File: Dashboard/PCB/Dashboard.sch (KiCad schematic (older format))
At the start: 97 parts, among them J3 LED, J4 MAIN_CONNECTOR, J5 BAOFENG_OUT, J6 Display, J7 PROGRAMMER, J8 MEM2051-00-195-00-A_REVC, SW1 SW_SPST, U1 STM32F767ZIT6, U2 MP2359DJ-LF-Z, U3 MP2359DJ-LF-Z, U4 AS4C1M16S-6TCN, U5 AT25SF128A-SHB-T, U6 MP2332H, U7 MCP2561-E-SN, U8 MCP2561-E-SN, Y1 Crystal_GND24

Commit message: Remove unnecessary files
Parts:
- removed J8: MEM2051-00-195-00-A_REVC, SDCARD:GCT_MEM2051-00-195-00-A_REVC, symbol MEM2051-00-195-00-A_REVC:MEM2051-00-195-00-A_REVC
- removed R19, R20, R21, R22: 47K, Resistor_SMD:R_0805_2012Metric, symbol Device:R
- added U?: ESP-12S, ESP-12S, symbol ESP-12S:ESP-12S
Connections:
- wire segments 405 -> 388
- no-connect marks 62 -> 70
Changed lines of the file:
@@
 	10950 13500 11050 13600
 Entry Wire Line
-	20500 5400 20600 5500
-Entry Wire Line
 	14550 12400 14650 12500
 $Comp
@@
 	12750 12300 12750 11700
 Connection ~ 12750 11700
-$Comp
-L power:+3.3V #PWR061
-U 1 1 61E60003
-P 13350 9250
-F 0 "#PWR061" H 13350 9100 50  0001 C CNN
-F 1 "+3.3V" H 13365 9423 50  0000 C CNN
-F 2 "" H 13350 9250 50  0001 C CNN
-F 3 "" H 13350 9250 50  0001 C CNN
-	1    13350 9250
-	-1   0    0    -1
-$EndComp
-$Comp
-L power:GND #PWR062
-U 1 1 61E60BC0
-P 13350 9950
-F 0 "#PWR062" H 13350 9700 50  0001 C CNN
-F 1 "GND" H 13355 9777 50  0000 C CNN
-F 2 "" H 13350 9950 50  0001 C CNN
-F 3 "" H 13350 9950 50  0001 C CNN
-	1    13350 9950
-	-1   0    0    -1
-$EndComp
-Wire Wire Line
-	13050 9950 13350 9950
-Wire Wire Line
-	13350 9250 13050 9250
-Entry Wire Line
-	13900 9650 14000 9750
-Entry Wire Line
-	13900 9750 14000 9850
-Entry Wire Line
-	13900 9350 14000 9450
-NoConn ~ 13050 9450
-NoConn ~ 13050 9550
-Entry Wire Line
-	13900 9850 14000 9950
-Text Label 13100 9350 0    50   ~ 0
-SD_MISO
-Text Label 13100 9850 0    50   ~ 0
-SD_SCLK
-Text Label 13100 9750 0    50   ~ 0
-SD_MOSI
-Text Label 13150 9650 0    50   ~ 0
-SD_CS
-$Comp
-L power:GND #PWR060
-U 1 1 61F62558
-P 13050 10250
-F 0 "#PWR060" H 13050 10000 50  0001 C CNN
-F 1 "GND" H 13055 10077 50  0000 C CNN
-F 2 "" H 13050 10250 50  0001 C CNN
-F 3 "" H 13050 10250 50  0001 C CNN
-	1    13050 10250
-	1    0    0    -1
-$EndComp
 Wire Wire Line
 	15200 12500 14650 12500
@@
 Entry Wire Line
 	13150 1850 13050 1950
-$Comp
-L Device:R R22
-U 1 1 6240A074
-P 13900 9050
-F 0 "R22" H 13970 9096 50  0000 L CNN
-F 1 "47K" H 13970 9005 50  0000 L CNN
-F 2 "Resistor_SMD:R_0805_2012Metric" V 13830 9050 50  0001 C CNN
-F 3 "~" H 13900 9050 50  0001 C CNN
-	1    13900 9050
-	1    0    0    -1
-$EndComp
-$Comp
-L Device:R R21
-U 1 1 6249BF7E
-P 13800 9050
-F 0 "R21" H 13870 9096 50  0000 L CNN
-F 1 "47K" H 13870 9005 50  0000 L CNN
-F 2 "Resistor_SMD:R_0805_2012Metric" V 13730 9050 50  0001 C CNN
-F 3 "~" H 13800 9050 50  0001 C CNN
-	1    13800 9050
-	1    0    0    -1
-$EndComp
-$Comp
-L Device:R R20
-U 1 1 624ABC5A
-P 13700 9050
-F 0 "R20" H 13770 9096 50  0000 L CNN
-F 1 "47K" H 13770 9005 50  0000 L CNN
-F 2 "Resistor_SMD:R_0805_2012Metric" V 13630 9050 50  0001 C CNN
-F 3 "~" H 13700 9050 50  0001 C CNN
-	1    13700 9050
-	1    0    0    -1
-$EndComp
-$Comp
-L Device:R R19
-U 1 1 624ABC60
-P 13600 9050
-F 0 "R19" H 13670 9096 50  0000 L CNN
-F 1 "47K" H 13670 9005 50  0000 L CNN
-F 2 "Resistor_SMD:R_0805_2012Metric" V 13530 9050 50  0001 C CNN
-F 3 "~" H 13600 9050 50  0001 C CNN
-	1    13600 9050
-	1    0    0    -1
-$EndComp
-Wire Wire Line
-	13900 9200 13900 9350
-Wire Wire Line
-	13900 8900 13800 8900
-Connection ~ 13700 8900
-Wire Wire Line
-	13700 8900 13600 8900
-Connection ~ 13800 8900
-Wire Wire Line
-	13800 8900 13700 8900
-$Comp
-L power:+3.3V #PWR063
-U 1 1 62568F6D
-P 13600 8900
-F 0 "#PWR063" H 13600 8750 50  0001 C CNN
-F 1 "+3.3V" H 13615 9073 50  0000 C CNN
-F 2 "" H 13600 8900 50  0001 C CNN
-F 3 "" H 13600 8900 50  0001 C CNN
-	1    13600 8900
-	1    0    0    -1
-$EndComp
-Connection ~ 13600 8900
-Wire Bus Line
-	14000 9950 14550 9950
-Connection ~ 14550 9950
 NoConn ~ 12350 1850
 NoConn ~ 12350 2050
 NoConn ~ 12350 2150
 NoConn ~ 13200 7850
-$Comp
-L MEM2051-00-195-00-A_REVC:MEM2051-00-195-00-A_REVC J8
-U 1 1 617876F8
-P 12850 9750
-F 0 "J8" H 13480 9796 50  0000 L CNN
-F 1 "MEM2051-00-195-00-A_REVC" H 13480 9705 50  0000 L CNN
-F 2 "SDCARD:GCT_MEM2051-00-195-00-A_REVC" H 12850 9750 50  0001 L BNN
-F 3 "" H 12850 9750 50  0001 L BNN
-F 4 "GCT" H 12850 9750 50  0001 L BNN "MANUFACTURER"
-	1    12850 9750
-	-1   0    0    -1
-$EndComp
-Wire Wire Line
-	13050 9650 13800 9650
-Wire Wire Line
-	13050 9350 13900 9350
-Wire Wire Line
-	13050 9750 13700 9750
-Wire Wire Line
-	13050 9850 13600 9850
-Wire Wire Line
-	13800 9200 13800 9650
-Connection ~ 13800 9650
-Wire Wire Line
-	13800 9650 13900 9650
-Wire Wire Line
-	13700 9200 13700 9750
-Connection ~ 13700 9750
-Wire Wire Line
-	13700 9750 13900 9750
-Wire Wire Line
-	13600 9200 13600 9850
-Connection ~ 13600 9850
-Wire Wire Line
-	13600 9850 13900 9850
-Wire Wire Line
-	13050 10150 13900 10150
-Wire Bus Line
-	14000 9950 14000 10250
-Connection ~ 14000 9950
-Entry Wire Line
-	13900 10150 14000 10250
-Text Label 13100 10150 0    50   ~ 0
-SD_CARD_DETECT
 Entry Wire Line
 	14550 1300 14650 1400
@@
 	4550 14850 4550 14750
 Connection ~ 4550 14850
-Wire Notes Line
-	900  800  3800 800
-Text Notes 1150 750  2    50   ~ 0
+Text Notes 1050 700  2    50   ~ 0
 Power\n
 Wire Notes Line
-	3800 4200 900  4200
-Wire Notes Line
-	900  800  900  4200
-Wire Notes Line
-	3800 800  3800 4200
-Wire Notes Line
 	4300 5300 9050 5300
 Wire Notes Line
@@
 Wire Wire Line
 	4550 6750 4550 6900
+$Comp
+L ESP-12S:ESP-12S U?
+U 1 1 61B531D3
+P 10550 7550
+F 0 "U?" H 10550 8417 50  0000 C CNN
+F 1 "ESP-12S" H 10550 8326 50  0000 C CNN
+F 2 "ESP-12S" H 10550 7550 50  0001 L BNN
+F 3 "" H 10550 7550 50  0001 L BNN
+F 4 "IC-14115" H 10550 7550 50  0001 L BNN "PROD_ID"
+	1    10550 7550
+	1    0    0    -1
+$EndComp
+NoConn ~ 10950 7150
+NoConn ~ 10950 7250
+NoConn ~ 10950 7350
+NoConn ~ 10950 7450
+NoConn ~ 10950 7550
+NoConn ~ 10950 7650
+NoConn ~ 10950 7750
+NoConn ~ 10950 7850
+NoConn ~ 10950 7950
+NoConn ~ 10950 8050
 Wire Bus Line
 	13150 1350 13150 1550
 Wire Bus Line
-	14000 9450 14000 9950
-Wire Bus Line
 	14200 7350 14200 7950
 Wire Bus Line
@@
 	13150 1550 13150 2250
 Wire Bus Line
-	14550 7950 14550 9950
-Wire Bus Line
 	14550 1550 14550 7950
 Wire Bus Line
 	10950 11400 10950 14000
 Wire Bus Line
-	14550 9950 14550 14000
-Wire Bus Line
 	13350 11600 13350 14000
+Wire Bus Line
+	14550 7950 14550 14000
+$Comp
+L power:+3.3V #PWR?
+U 1 1 61E1DAA6
+P 10050 6950
+F 0 "#PWR?" H 10050 6800 50  0001 C CNN
+F 1 "+3.3V" H 10065 7123 50  0000 C CNN
+F 2 "" H 10050 6950 50  0001 C CNN
+F 3 "" H 10050 6950 50  0001 C CNN
+	1    10050 6950
+	1    0    0    -1
+$EndComp
 $EndSCHEMATC

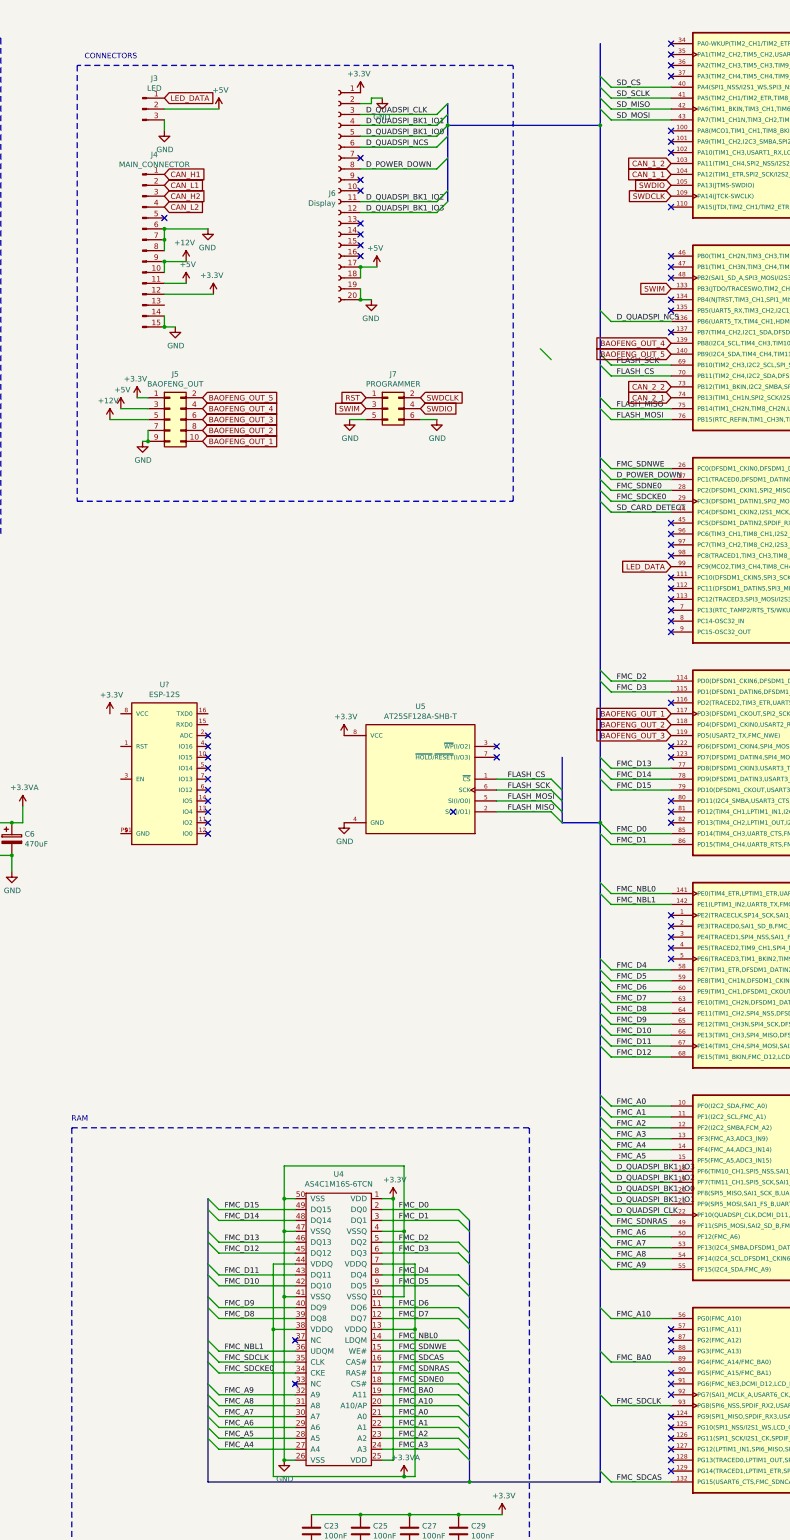
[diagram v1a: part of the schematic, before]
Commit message: ADD new pcb files
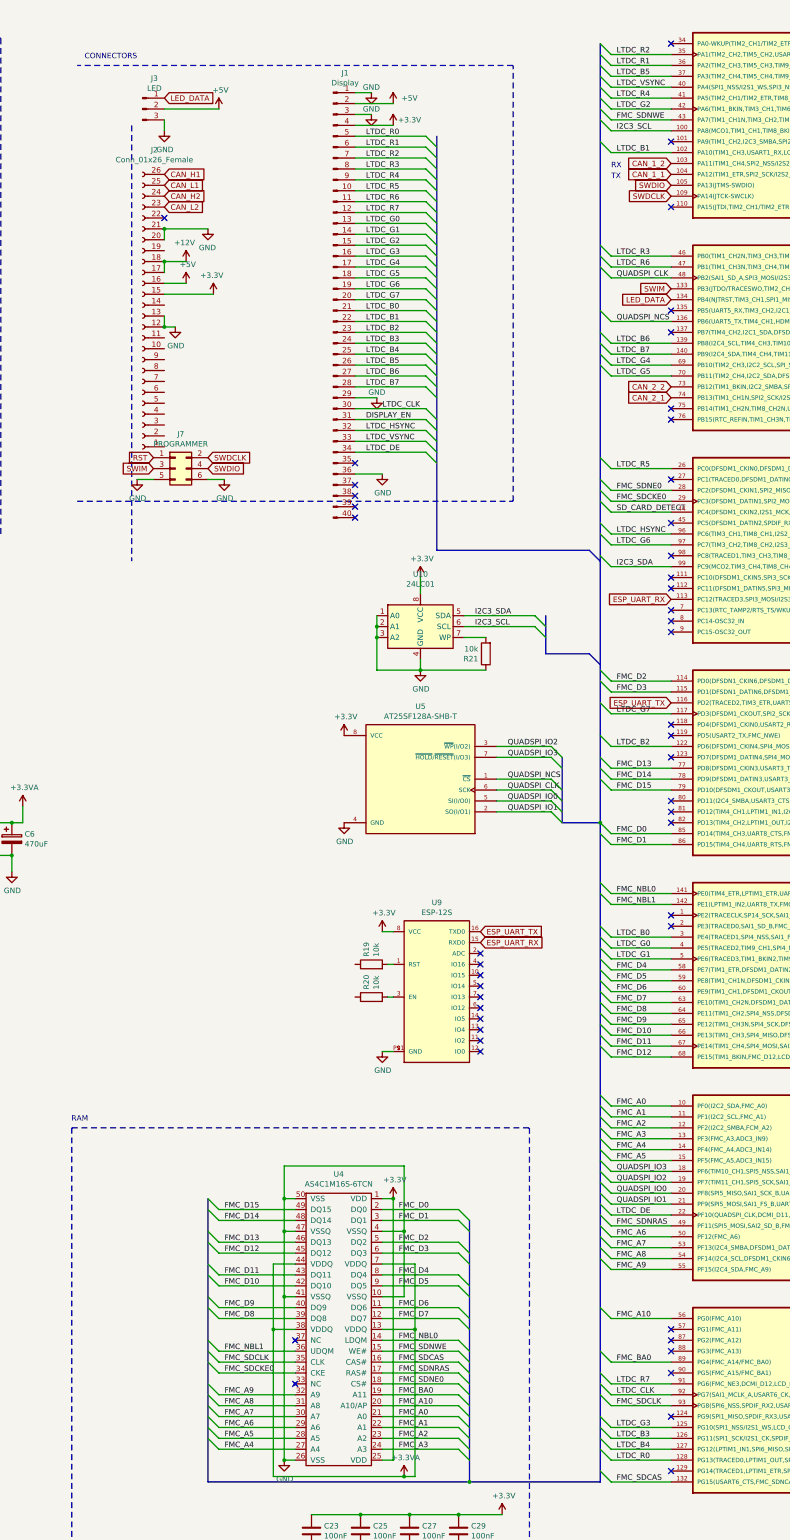
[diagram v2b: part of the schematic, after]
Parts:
- removed J4: MAIN_CONNECTOR, Connector:DT13, symbol Connector:Conn_01x15_Male
- removed J5: BAOFENG_OUT, Connector_PinSocket_2.54mm:PinSocket_2x05_P2.54mm_Vertical, symbol Connector_Generic:Conn_02x05_Odd_Even
- removed J6: Display, Connector_FFC-FPC:Hirose_FH12-20S-0.5SH_1x20-1MP_P0.50mm_Horizontal, symbol Connector:Conn_01x20_Female
- added J1: Display, Connector_FFC-FPC:Hirose_FH12-40S-0.5SH_1x40-1MP_P0.50mm_Horizontal, symbol Connector:Conn_01x40_Male
- added J2: Conn_01x26_Female, Konektor:64734231, symbol Connector:Conn_01x26_Female
- added R19, R20, R21: 10k, Resistor_SMD:R_0805_2012Metric, symbol Device:R
- added U10: 24LC01, Package_DIP:DIP-8_W7.62mm_Socket_LongPads, symbol Memory_EEPROM:24LC01
- U9: renamed from U?; footprint ESP-12S -> ESP-12S:ESP-12S
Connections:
- net D_QUADSPI_BK1_IO2 is gone; now on net QUADSPI_IO2: U1.19 (PF7(TIM11_CH1,SPI5_SCK,SAI1_MCK_B,UART7_TX,QUADSPI_BK1_IO2,ADC3_IN5))
- net D_QUADSPI_BK1_IO3 is gone; now on net QUADSPI_IO3: U1.18 (PF6(TIM10_CH1,SPI5_NSS,SAI1_SD_B,UART7_RX,QUADSPI_BK1_IO3,ADC3_IN4))
- net SD_MOSI is gone; now on net FMC_SDNWE: U1.43 (PA7(TIM1_CH1N,TIM3_CH2,TIM8_CH1N,SPI1_MOSI/I2S1_SD,SPI6_MOSI,TIM14_CH1,ETH_MII_RX_DV/ETH_RMII_CRS_DV,FMC_SDNWE))
- net +12V: now also J2.17 (Pin_17), J2.18 (Pin_18)
- net +3V3: now also U9.8 (VCC), J1.4 (Pin_4), J2.15 (Pin_15), U10.8 (VCC)
- net +5V: now also J1.2 (Pin_2), J2.16 (Pin_16)
- net CAN_H1: now also J2.26 (Pin_26)
- net CAN_H2: now also J2.24 (Pin_24)
- net CAN_L1: now also J2.25 (Pin_25)
- net CAN_L2: now also J2.23 (Pin_23)
- net FMC_SDNWE: no longer U1.26 (PC0(DFSDM1_CKIN0,DFSDM1_DATIN4,SAI2_FS_B,OTG_HS_ULPI_STP,FMC_SDNWE,LCD_R5,ADC1_IN10,ADC2_IN10,ADC3_IN10))
- net GND: now also U9.9 (GND), U9.P$1 (GND), J1.1 (Pin_1), J1.29 (Pin_29), J1.3 (Pin_3), J1.36 (Pin_36), J2.12 (Pin_12), J2.13 (Pin_13), J2.20 (Pin_20), J2.21 (Pin_21), R21.1, U10.1 (A0), U10.2 (A1), U10.3 (A2), U10.4 (GND)
- net LED_DATA: now also U1.134 (PB4(NJTRST,TIM3_CH1,SPI1_MISO,SPI3_MISO,SPI2_NSS/I2S2_WS,SPI6_MISO,SDMMC2_D3,CAN3_TX,UART7_TX)); no longer U1.99 (PC9(MCO2,TIM3_CH4,TIM8_CH4,I2S3_SDA,I2S_CKIN,UART5_CTS,QUADSPI_BK1_IO0,LCD_G3,SDMMC12_D1,DCMI_D3,LCD_B2))
- net I2C3_SCL: now reaches U1.100 (PA8(MCO1,TIM1_CH1,TIM8_BKIN2,I2C3_SCL,USART1_CK,OTG_FS_SOF,CAN3_RX,UART7_RX,LCD_B3,LCD_R6))
- net I2C3_SCL: now also U10.6 (SCL)
- net LTDC_B1: now reaches U1.102 (PA10(TIM1_CH3,USART1_RX,LCD_B4,OTG_FS_ID,MDIOS_MDIO,DCMI_D1,LCD_B1))
- net LTDC_B1: now also J1.22 (Pin_22)
- net LTDC_R2: now reaches U1.35 (PA1(TIM2_CH2,TIM5_CH2,USART2_RTS,UART4_RX,QUADSPI_BK1_IO3,SAI2_MCLK_B,ETH_MII_RX_CLK/ETH_RMII_REF_CLK,LCD_R2))
- net LTDC_R2: now also J1.7 (Pin_7)
- net LTDC_R1: now reaches U1.36 (PA2(TIM2_CH3,TIM5_CH3,TIM9_CH1,USART2_TX,SAI2_SCK_B,ETH_MDIO,MDIOS_MDIO,LCD_R1,ADC1_IN2,ADC2_IN2,ADC3_IN2,WKUP2))
- net LTDC_R1: now also J1.6 (Pin_6)
- net LTDC_B5: now reaches U1.37 (PA3(TIM2_CH4,TIM5_CH4,TIM9_CH2,USART2_RX,LCD_B2,OTG_HS_ULPI_D0,ETH_MII_COL,LCD_B5,ADC1_IN3,ADC2_IN3,ADC3_IN3))
- net LTDC_B5: now also J1.26 (Pin_26)
- net LTDC_R3: now reaches U1.46 (PB0(TIM1_CH2N,TIM3_CH3,TIM8_CH2N,DFSDM1_CKOUT,UART4_CTS,LCD_R3,OTG_HS_ULPI_D1,ETH_MII_RXD2,LCD_G1,ADC1_IN8,ADC2_IN8))
- net LTDC_R3: now also J1.8 (Pin_8)
- net LTDC_R6: now reaches U1.47 (PB1(TIM1_CH3N,TIM3_CH4,TIM8_CH3N,DFSDM1_DATIN1,LCD_R6,OTG_HS_ULPI_D2,ETH_MII_RXD3,LCD_G0,ADC1_IN9,ADC2_IN9))
- net LTDC_R6: now also J1.11 (Pin_11)
- net QUADSPI_CLK: now reaches U1.48 (PB2(SAI1_SD_A,SPI3_MOSI/I2S3_SD,QUADSPI_CLK,DFSDM1_CKIN1))
- net QUADSPI_CLK: now also U5.6 (SCK)
- net ESP_UART_RX: now reaches U1.113 (PC12(TRACED3,SPI3_MOSI/I2S3_SD,USART3_CK,UART5_TX,SDMMC1_CK,DCMI_D9))
- net ESP_UART_RX: now also U9.15 (RXD0)
- net LTDC_HSYNC: now reaches U1.96 (PC6(TIM3_CH1,TIM8_CH1,I2S2_MCK,DFSDM1_CKIN3,USART6_TX,TMC_NWAIT,SDMMC2_D6,SDMMC1_D6,DCMI_D0,LCD_HSYNC))
- net LTDC_HSYNC: now also J1.32 (Pin_32)
- net LTDC_G6: now reaches U1.97 (PC7(TIM3_CH2,TIM8_CH2,I2S3_MCK,DFSDM1_DATIN3,USART6_RX,FMC_NE1,SDMMC2_D7,SDMMC1_D7,DCMI_D1,LCD_G6))
- net LTDC_G6: now also J1.19 (Pin_19)
- net ESP_UART_TX: now reaches U1.116 (PD2(TRACED2,TIM3_ETR,UART5_RX,SDMMC1_CMD,DCMI_D11))
- net ESP_UART_TX: now also U9.16 (TXD0)
- net LTDC_B2: now reaches U1.122 (PD6(DFSDM1_CKIN4,SPI4_MOSI/I2S3_SD,SAI1_SD_A,USART2_RX,DFSDM1_DATIN1,SDMMC2_CK,FMC_NWAIT,DCMI_D10,LCD_B2))
- net LTDC_B2: now also J1.23 (Pin_23)
- net LTDC_B0: now reaches U1.3 (PE4(TRACED1,SPI4_NSS,SAI1_FS_A,DFSDM1_DATIN3,FMC_A20,DCMI_D4,LCD_B0))
- net LTDC_B0: now also J1.21 (Pin_21)
- net LTDC_G0: now reaches U1.4 (PE5(TRACED2,TIM9_CH1,SPI4_MISO,SAI1_SCK_A,DFSDM1_CKIN3,FMC_A21,DCMI_D6,LCD_G0))
- net LTDC_G0: now also J1.13 (Pin_13)
- net LTDC_G1: now reaches U1.5 (PE6(TRACED3,TIM1_BKIN2,TIM9_CH2,SPI4_MOSI,SAI1_SD_A,SAI2_MCLK_B,FMC_A22,DCMI_D7,LCD_G1))
- net LTDC_G1: now also J1.14 (Pin_14)
- net LTDC_G3: now reaches U1.125 (PG10(SPI1_NSS/I2S1_WS,LCD_G3,SAI2_SD_B,SDMMC2_D1,FMC_NE3,DCMI_D2,LCD_B2))
- net LTDC_G3: now also J1.16 (Pin_16)
- net LTDC_B3: now reaches U1.126 (PG11(SPI1_SCK/I2S1_CK,SPDIF_RX0,SDMMC2_D2,ETH_MII_TX_EN/ETH_RMII_TX_EN,DCMI_D3,LCD_B3))
- net LTDC_B3: now also J1.24 (Pin_24)
- net LTDC_B4: now reaches U1.127 (PG12(LPTIM1_IN1,SPI6_MISO,SPDIF_RX1,USART6_RTS,LCD_B4,SDMMC2_D3,FMC_NE4,LCD_B1))
- net LTDC_B4: now also J1.25 (Pin_25)
- net LTDC_R0: now reaches U1.128 (PG13(TRACED0,LPTIM1_OUT,SPI6_SCK,USART6_CTS,ETH_MII_TXD0/ETH_RMII_TXD0,FMC_A24,LCD_R0))
- net LTDC_R0: now also J1.5 (Pin_5)
- net LTDC_R7: now reaches U1.91 (PG6(FMC_NE3,DCMI_D12,LCD_R7)))
- net LTDC_R7: now also J1.12 (Pin_12)
- net LTDC_CLK: now reaches U1.92 (PG7(SAI1_MCLK_A,USART6_CK,FMC_INT,DCMII_D13,LCD_CLK))
- net LTDC_CLK: now also J1.30 (Pin_30)
- net QUADSPI_IO2: now reaches U5.3 (~WP~(I/O2))
- net QUADSPI_IO3: now reaches U5.7 (~HOLD~/~RESET~(I/O3))
- net at U9.1 (RST): now also R19.2
- net at U9.3 (EN): now also R20.2
- net BAOFENG_OUT_1 renamed LTDC_G7
- net LTDC_G7: now also J1.20 (Pin_20)
- net BAOFENG_OUT_2: no longer names the net of U1.118 (PD4(DFSDM1_CKIN0,USART2_RTS,FMC_NOE))
- net BAOFENG_OUT_3: no longer names the net of U1.119 (PD5(USART2_TX,FMC_NWE))
- net BAOFENG_OUT_4 renamed LTDC_B6
- net LTDC_B6: now also J1.27 (Pin_27)
- net BAOFENG_OUT_5 renamed LTDC_B7
- net LTDC_B7: now also J1.28 (Pin_28)
- net D_POWER_DOWN: no longer names the net of U1.27 (PC1(TRACED0,DFSDM1_DATIN0,SAI2_MOSI/I2S2_SD,SAI1_SD_A,DFSDM1_CKIN4,ETH_MDC,MDIOS_MDC,ADC1_IN11,ADC2_IN11,ADC3_IN11,RTC_TAMP3))
- net D_QUADSPI_BK1_IO0 renamed QUADSPI_IO0
- net QUADSPI_IO0: now also U5.5 (SI(I/O0))
- net D_QUADSPI_BK1_IO1 renamed QUADSPI_IO1
- net QUADSPI_IO1: now also U5.2 (SO(I/O1))
- net D_QUADSPI_CLK renamed LTDC_DE
- net LTDC_DE: now also J1.34 (Pin_34)
- net D_QUADSPI_NCS renamed QUADSPI_NCS
- net QUADSPI_NCS: now also U5.1 (~CS)
- net FLASH_CS renamed LTDC_G5
- net LTDC_G5: now also J1.18 (Pin_18); no longer U5.1 (~CS)
- net FLASH_MISO: no longer names the net of U1.75 (PB14(TIM1_CH2N,TIM8_CH2N,USART1_TX,SPI2_MISO,DFSDM1_DATIN2,USART3_RTS,UART4_RTS,TIM12_CH1,SDMMC2_D0,OTG_HS_DM))
- net FLASH_MISO: no longer U5.2 (SO(I/O1))
- net FLASH_MOSI: no longer names the net of U1.76 (PB15(RTC_REFIN,TIM1_CH3N,TIM8_CH3N,USART1_RX,SPI2_MOSI/I2S2_SD,DFSDM1_CKIN2,UART4_CTS,TIM12_CH2,SDMMC2_D1,OTG_HS_DP))
- net FLASH_MOSI: no longer U5.5 (SI(I/O0))
- net FLASH_SCK renamed LTDC_G4
- net LTDC_G4: now also J1.17 (Pin_17); no longer U5.6 (SCK)
- net SD_CS renamed LTDC_VSYNC
- net LTDC_VSYNC: now also J1.33 (Pin_33)
- net SD_MISO renamed LTDC_G2
- net LTDC_G2: now also J1.15 (Pin_15)
- net SD_SCLK renamed LTDC_R4
- net LTDC_R4: now also J1.9 (Pin_9)
- new net: R21.2, U10.7 (WP)
- new net DISPLAY_EN: J1.31 (Pin_31)
- new net I2C3_SDA: U1.99 (PC9(MCO2,TIM3_CH4,TIM8_CH4,I2S3_SDA,I2S_CKIN,UART5_CTS,QUADSPI_BK1_IO0,LCD_G3,SDMMC12_D1,DCMI_D3,LCD_B2)), U10.5 (SDA)
- new net LTDC_R5: J1.10 (Pin_10), U1.26 (PC0(DFSDM1_CKIN0,DFSDM1_DATIN4,SAI2_FS_B,OTG_HS_ULPI_STP,FMC_SDNWE,LCD_R5,ADC1_IN10,ADC2_IN10,ADC3_IN10))
- no-connect marks 70 -> 47
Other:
- note added: "RX\n"
- note added: "TX\n"
- moved on the sheet: J7, U9
